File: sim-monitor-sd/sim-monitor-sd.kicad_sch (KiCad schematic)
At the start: 20 parts, among them J1 A-DF_09_A_KG-T4S, U1 ESP32-DEVKITC-32D, U2 TLP291-4, U3 TLP291-4, U4 MP2315SGJ-Z

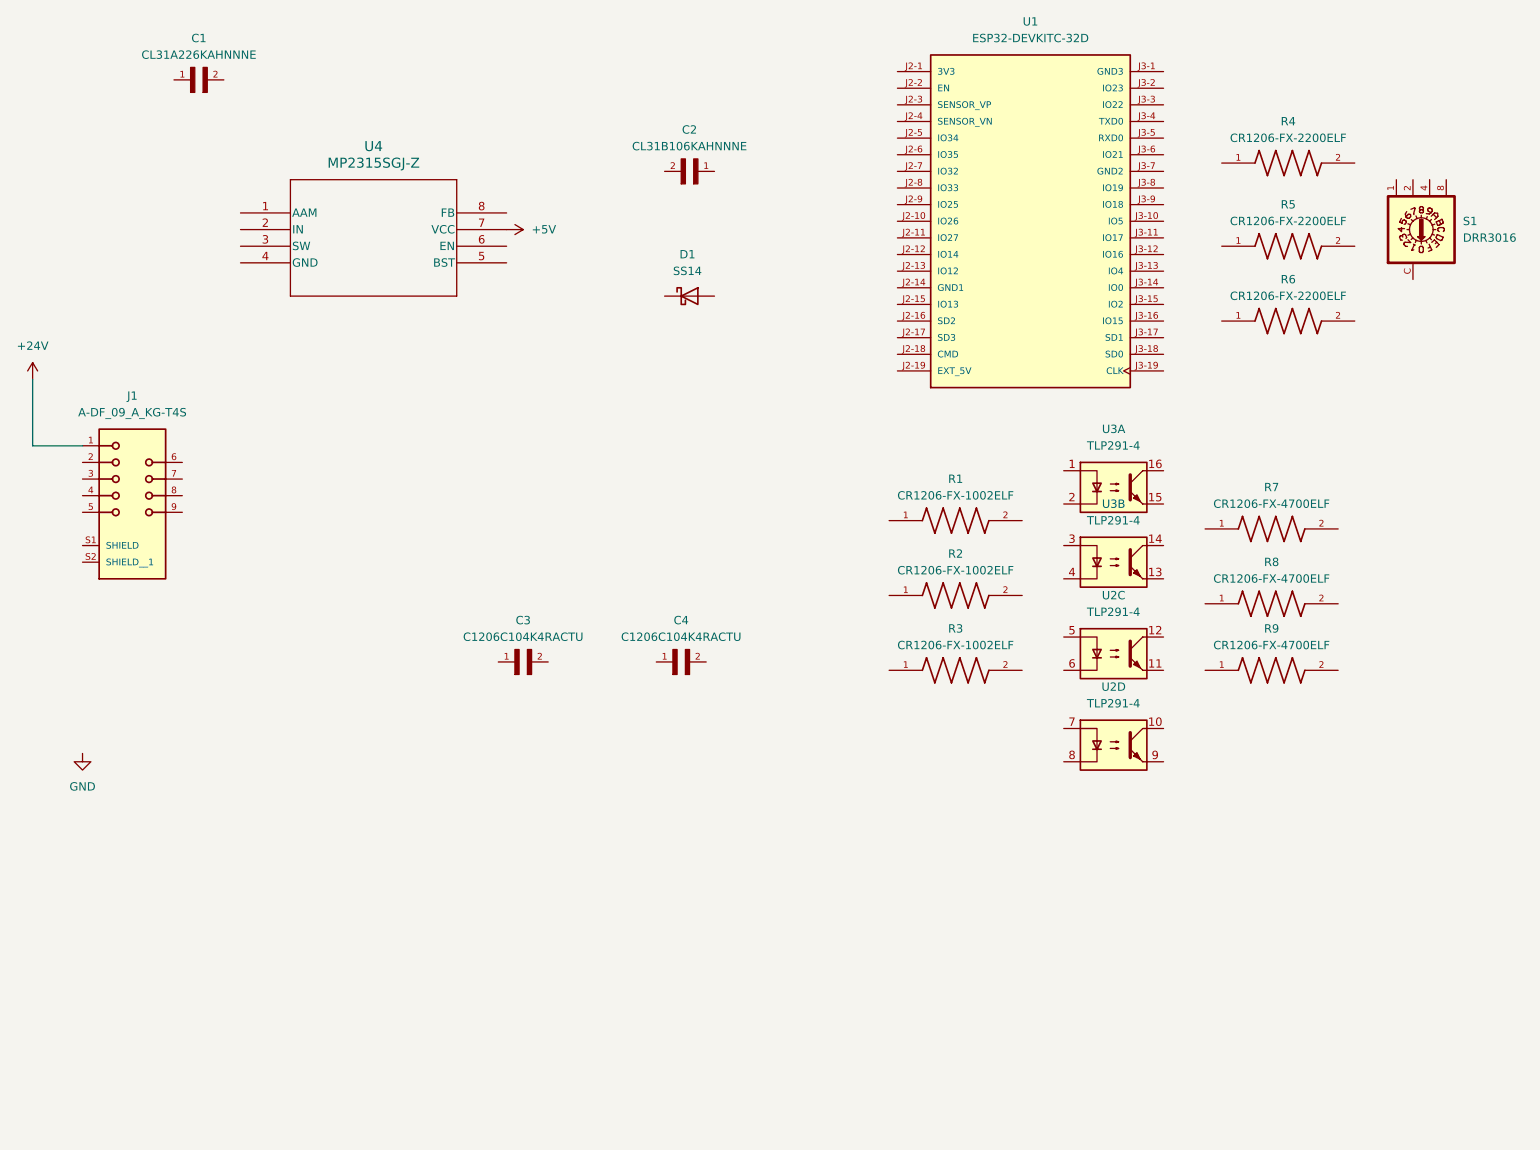
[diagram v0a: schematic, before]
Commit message: 6Mar
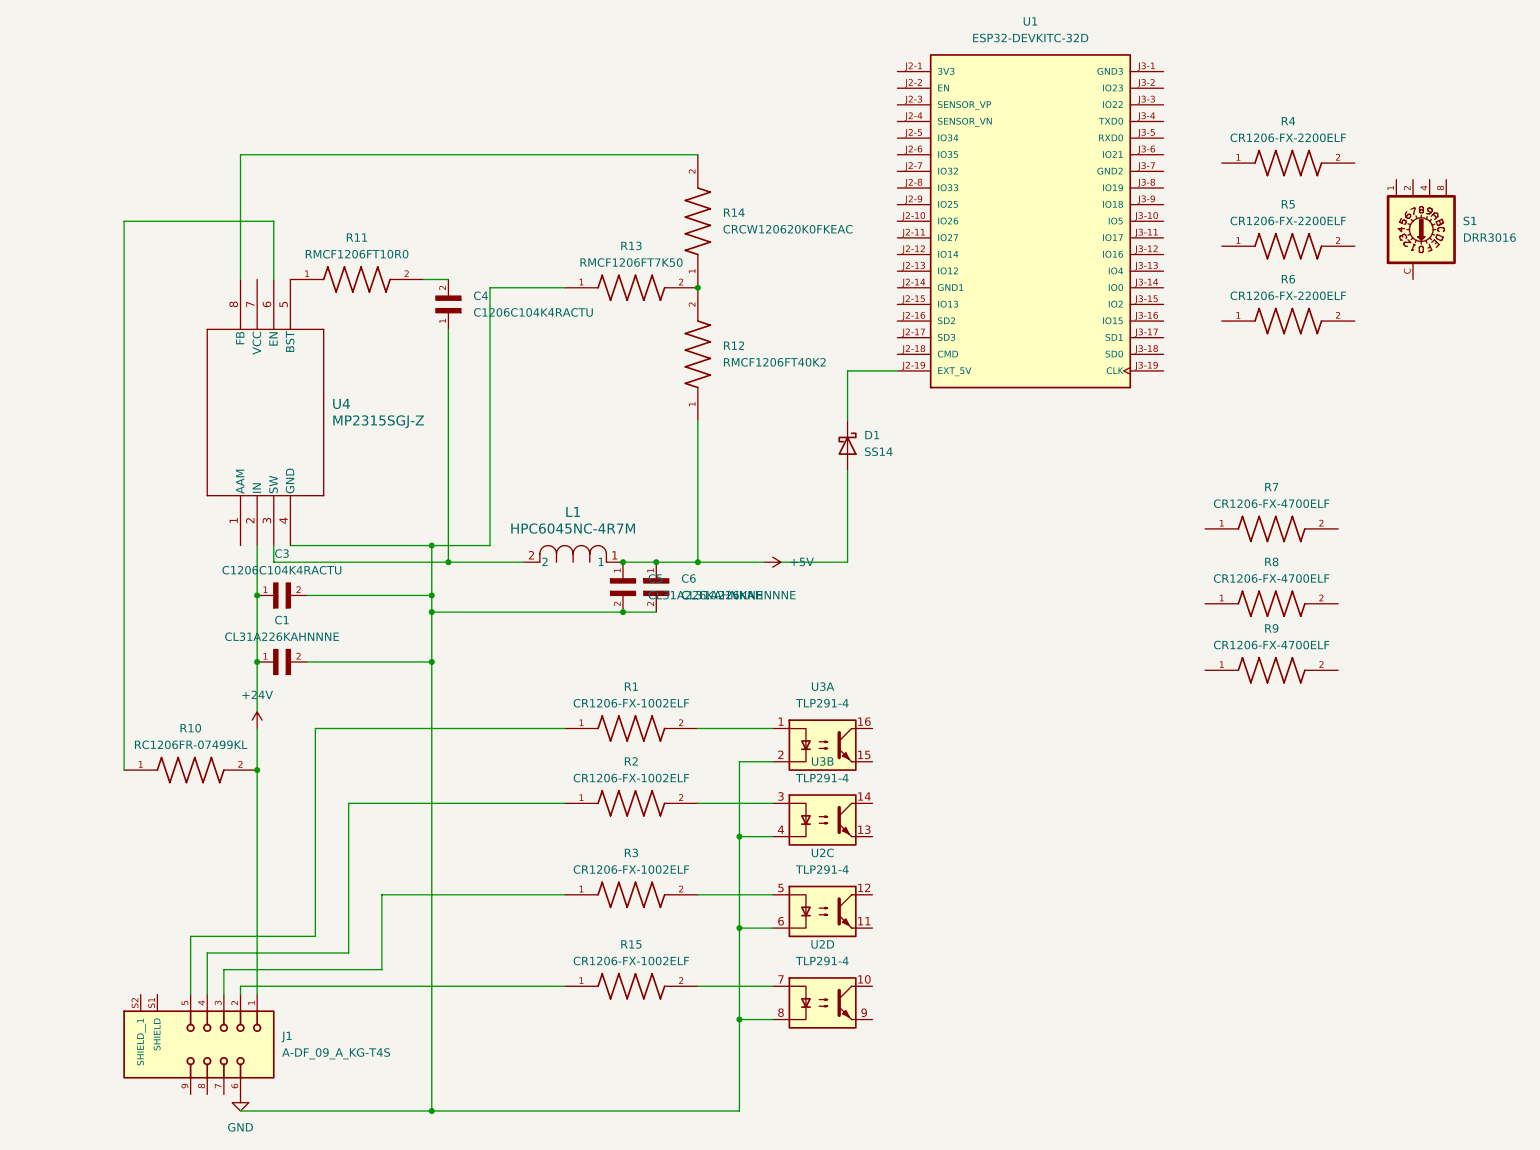
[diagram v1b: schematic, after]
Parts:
- removed C2: CL31B106KAHNNNE, CL31B106KAHNNNE:CAPC3216X180N, symbol CL31B106KAHNNNE:CL31B106KAHNNNE
- added C5, C6: CL31A226KAHNNNE, CL31A226KAHNNNE:CAPC3216X180N, symbol CL31A226KAHNNNE:CL31A226KAHNNNE
- added L1: HPC6045NC-4R7M, IND_HPC6045NC_TTA, symbol 2025-03-06_05-32-12:HPC6045NC-4R7M
- added R10: RC1206FR-07499KL, RC1206FR-07499KL:RESC3116X65N, symbol RC1206FR-07499KL:RC1206FR-07499KL
- added R11: RMCF1206FT10R0, RMCF1206FT10R0:RESC3216X70N, symbol RMCF1206FT10R0:RMCF1206FT10R0
- added R12: RMCF1206FT40K2, RMCF1206FT40K2:RESC3216X70N, symbol RMCF1206FT40K2:RMCF1206FT40K2
- added R13: RMCF1206FT7K50, RMCF1206FT7K50:RESC3216X70N, symbol RMCF1206FT7K50:RMCF1206FT7K50
- added R14: CRCW120620K0FKEAC, CRCW120620K0FKEAC:RESC3015X65N, symbol CRCW120620K0FKEAC:CRCW120620K0FKEAC
- added R15: CR1206-FX-1002ELF, CR1206-FX-1002ELF:RESC3216X75N, symbol CR1206-FX-1002ELF:CR1206-FX-1002ELF
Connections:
- net +24V: now also R10.2
- net +5V: now also C5.1, C6.1, L1.1, R12.1; no longer U4.7 (VCC)
- net GND: now also J1.6
- net at U1.J2-19 (EXT_5V): now also D1.1 (K)
- net at U4.2 (IN): now also C1.1, C3.1
- net at U4.3 (SW): now also C4.1, L1.2
- net at U4.4 (GND): now also C1.2, C3.2, U2.6, U2.8, U3.2, U3.4, C5.2, C6.2, R13.1
- net at U4.5 (BST): now also R11.1
- net at U4.6 (EN): now also R10.1
- net at U4.8 (FB): now also R14.2
- net at C4.2: now also R11.2
- net at U3.1: now also R1.2
- net at U2.5: now also R3.2
- net at R2.1: now also J1.4
- net at R2.2: now also U3.3
- net at J1.2: now also R15.1
- net at J1.3: now also R3.1
- net at J1.5: now also R1.1
- net at U2.7: now also R15.2
- new net: R12.2, R13.2, R14.1
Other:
- moved on the sheet: C1, C3, C4, D1, J1, R1, R2, R3, U2C, U2D, U3A, U3B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
